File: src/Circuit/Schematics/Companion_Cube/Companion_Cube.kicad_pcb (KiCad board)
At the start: 2 copper layers, 42.2 x 23.5 mm, 15 parts, among them CON1 AVR-ISP-6, IC1 ATTINY85-S, P1 CONN_11, U1 MINI-B_USB

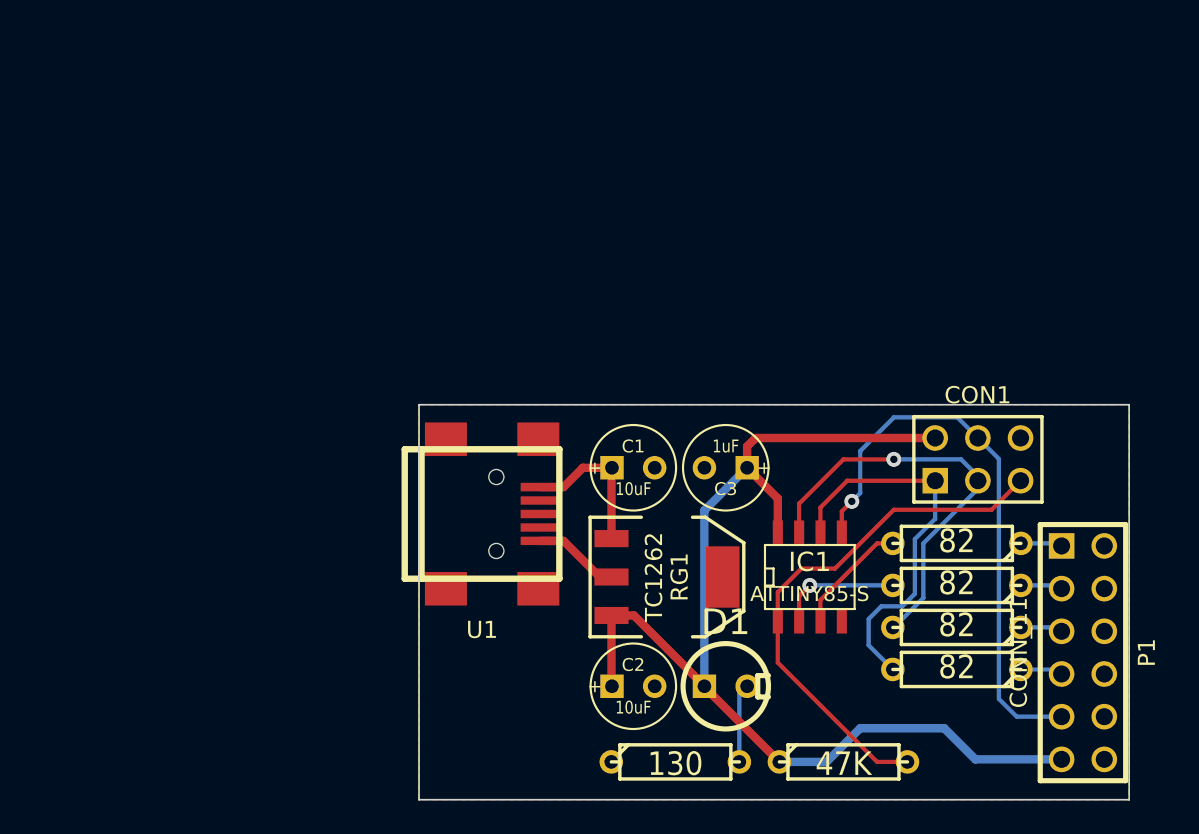
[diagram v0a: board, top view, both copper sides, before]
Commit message: Redesigning circuit board for new model
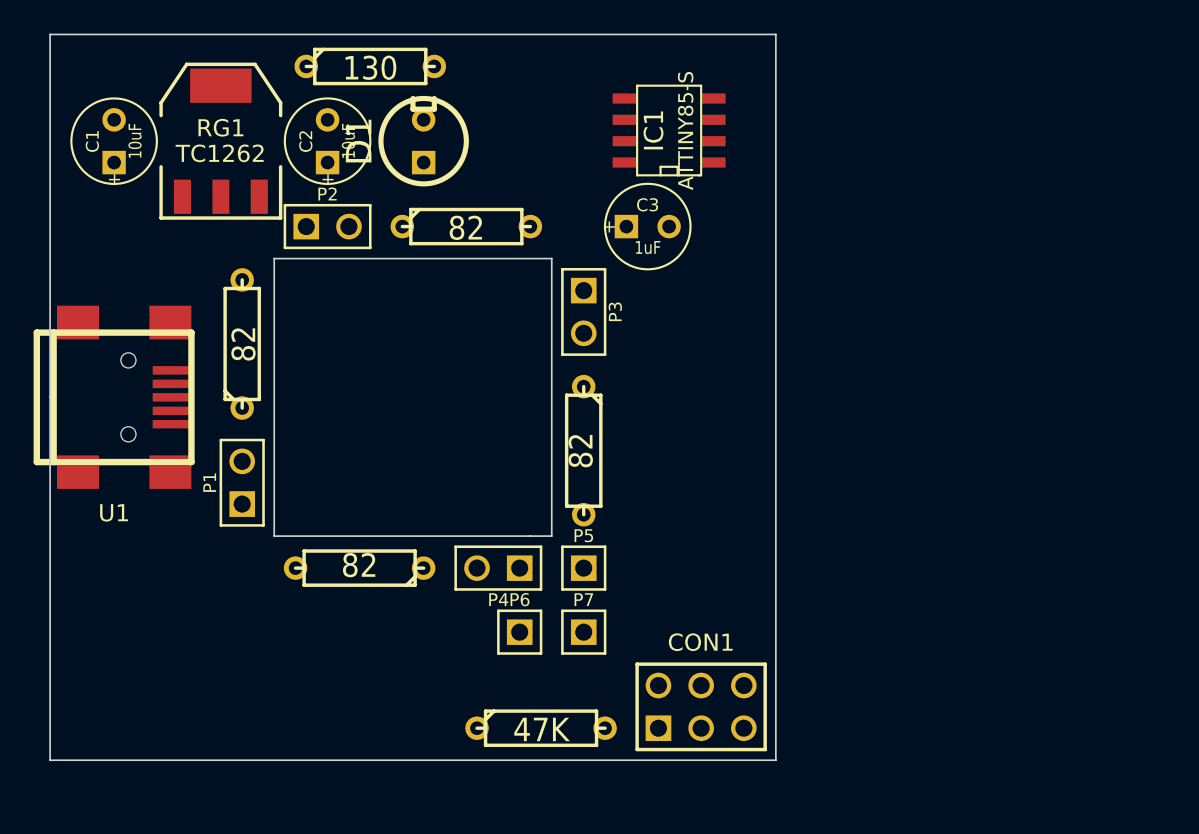
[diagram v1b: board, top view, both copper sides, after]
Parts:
- added P2: LED_3, PIN_ARRAY_2X1, F.Cu at (194.3, 120.7)
- added P3: LED_2, PIN_ARRAY_2X1, F.Cu at (209.6, 125.7)
- added P4: LED_1, PIN_ARRAY_2X1, F.Cu at (204.5, 141.0)
- added P5: CONN_1, PIN_ARRAY_1, F.Cu at (209.6, 141.0)
- added P6: CONN_1, PIN_ARRAY_1, F.Cu at (205.7, 144.8)
- added P7: CONN_1, PIN_ARRAY_1, F.Cu at (209.6, 144.8)
- P1: value CONN_11 -> LED_4; footprint pin_array_6x2 -> PIN_ARRAY_2X1
- moved P1 51.0 mm to (189.2, 135.9), turned to 90 degrees
- moved R1 46.7 mm to (189.2, 127.6), turned to 90 degrees
- moved R5 45.2 mm to (196.8, 111.1)
- moved R2 37.7 mm to (202.6, 120.7), turned to 0 degrees
- moved C2 37.2 mm to (194.3, 115.6), turned to 90 degrees
- moved RG1 37.1 mm to (188.0, 115.6), turned to 0 degrees
- moved D1 37.1 mm to (200.0, 115.6), turned to 90 degrees
- moved C1 36.5 mm to (181.6, 115.6), turned to 90 degrees
- moved R4 35.6 mm to (196.2, 141.0)
- moved IC1 27.9 mm to (214.6, 114.9), turned to 90 degrees
- moved R3 23.6 mm to (209.6, 134.0), turned to 270 degrees
- moved U1 23.0 mm to (181.6, 130.8)
- moved CON1 22.1 mm to (216.5, 149.2)
- moved R6 18.1 mm to (207.0, 150.5)
- moved C3 15.1 mm to (213.4, 120.7), turned to 0 degrees
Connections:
- CON1 pad 4: N-000005 (its old number) -> N-000003
- IC1 pad 5: N-000005 (its old number) -> N-000003
- P1 pad 1: N-000004 (its old number) -> GND
- P1 pad 2: GND -> N-0000012
- R1 pad 1: N-000001 -> N-0000012
- R2 pad 1: N-000002 (its old number) -> N-0000011
- R3 pad 1: N-000003 -> N-0000010
- R4 pad 1: N-000004 (its old number) -> N-000008
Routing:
- net VCC: track 67.6 -> 0.00 mm
- net N-000005 (its old number): track 33.8 -> 0.00 mm, vias 1 -> 0
- net N-000002: track 31.5 -> 0.00 mm
- net N-000006: track 25.0 -> 0.00 mm, vias 1 -> 0
- net N-000007: track 23.2 -> 0.00 mm
- net N-0000017: track 8.98 -> 0.00 mm
- net N-000005: track 7.37 -> 0.00 mm, vias 1 -> 0
- net N-000004: track 7.00 -> 0.00 mm
- net GND: track 5.14 -> 0.00 mm
- net N-000009: track 4.69 -> 0.00 mm
- net N-000001: track 2.53 -> 0.00 mm
- net N-000002 (its old number): track 2.52 -> 0.00 mm
- net N-000003: track 2.50 -> 0.00 mm
- net N-000004 (its old number): track 2.48 -> 0.00 mm
- removed copper zone on F.Cu, net GND
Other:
- board size 42.2 x 23.5 mm -> 43.2 x 43.2 mm
- board text removed: "Designed By Tyler Hackett 2014"
- board text removed: "TASH"
